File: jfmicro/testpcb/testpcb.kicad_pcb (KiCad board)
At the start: 2 copper layers, 60.3 x 66.7 mm, 32 parts, among them J1 Type C, K1 KEYSW, K2 KEYSW, K3 KEYSW, K4 KEYSW, K5 KEYSW, K6 KEYSW, SW1 SW_PUSH, SW2 Rotary_Encoder_Switch, U1 ATMEGA32U4, Y1 16MHz

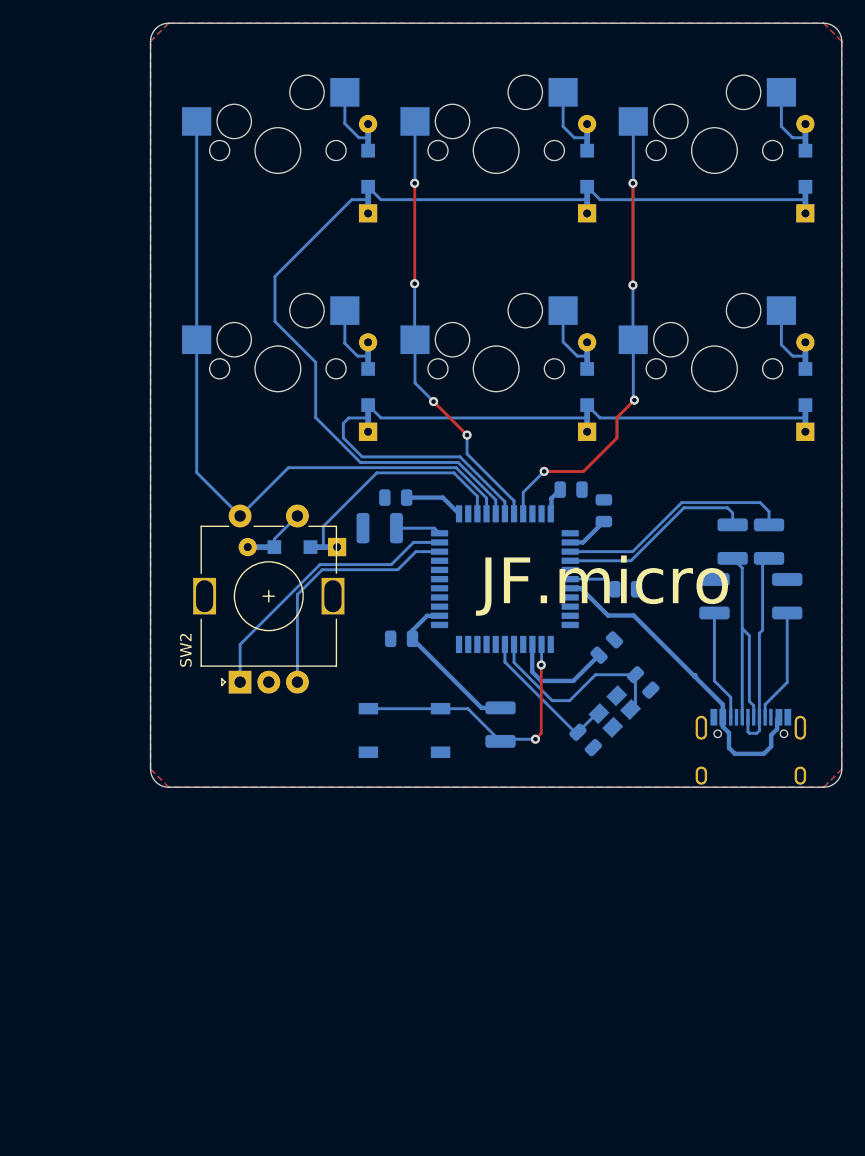
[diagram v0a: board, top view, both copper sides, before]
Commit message: micro revision two and more comps
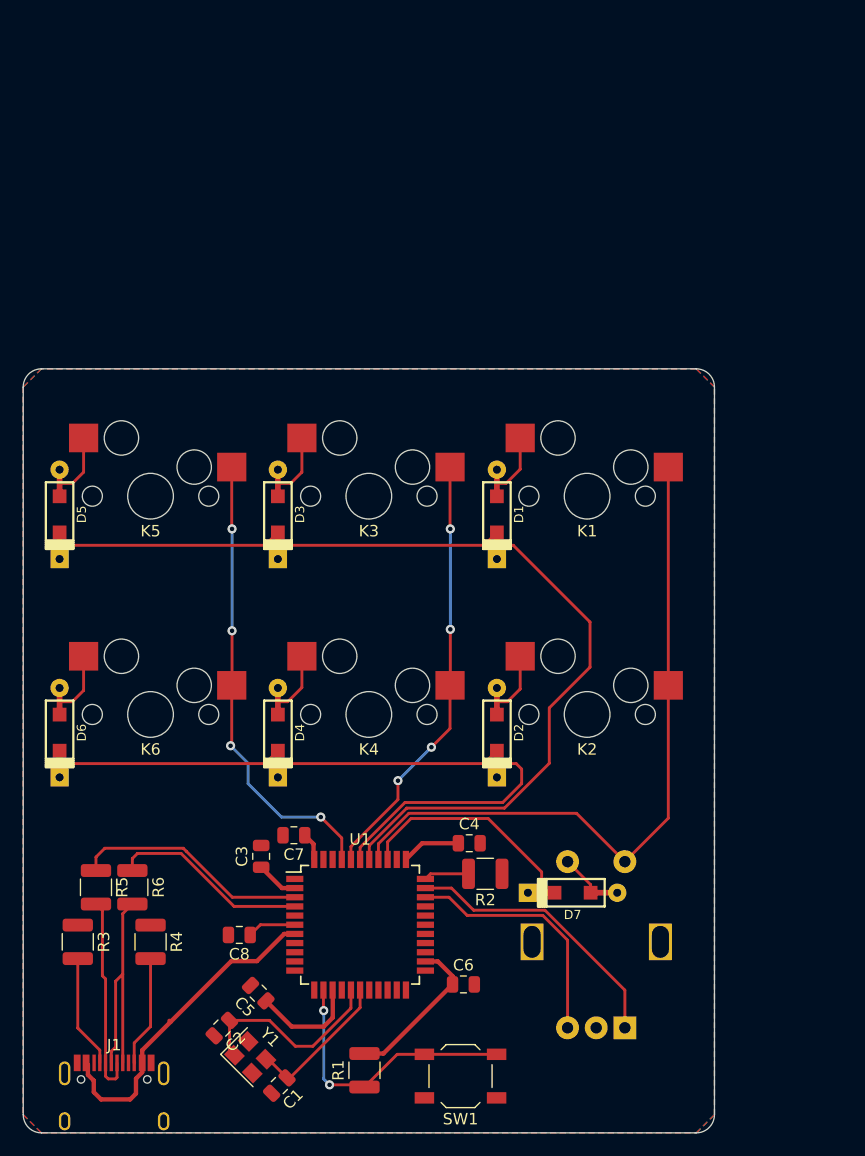
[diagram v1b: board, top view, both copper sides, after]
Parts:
- C1, C2, C3, C4, C5, C6, C7, C8, D1, D2, D3, D4, D5, D6, D7, J1, R1, R2, R3, R4, R5, R6, SW1, U1, Y1: moved to F.Cu
- K1, K2, K3, K4, K5, K6, SW2: moved to B.Cu
- moved D5 71.7 mm to (38.1, 65.1)
- moved D6 71.7 mm to (38.1, 84.1)
- moved R3 68.9 mm to (39.7, 102.4)
- moved R5 66.0 mm to (41.3, 97.6)
- moved J1 63.2 mm to (42.9, 120.7), turned to 0 degrees
- moved R6 60.5 mm to (44.5, 97.6)
- moved K5 57.7 mm to (46.0, 63.5), turned to 180 degrees
- moved K6 57.7 mm to (46.0, 82.5), turned to 180 degrees
- moved R4 57.7 mm to (46.0, 102.4)
- moved C2 47.6 mm to (52.3, 109.9), turned to 225 degrees
- moved C8 45.2 mm to (53.8, 101.8), turned to 180 degrees
- moved Y1 43.8 mm to (54.7, 112.5), turned to 315 degrees
- moved C5 42.8 mm to (55.4, 106.9), turned to 135 degrees
- moved C3 42.5 mm to (55.7, 94.9)
- moved SW2 41.5 mm to (84.9, 102.4)
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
